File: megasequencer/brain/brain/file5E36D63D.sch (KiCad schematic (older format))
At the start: 24 parts, among them U3 TL074, U4 TL072

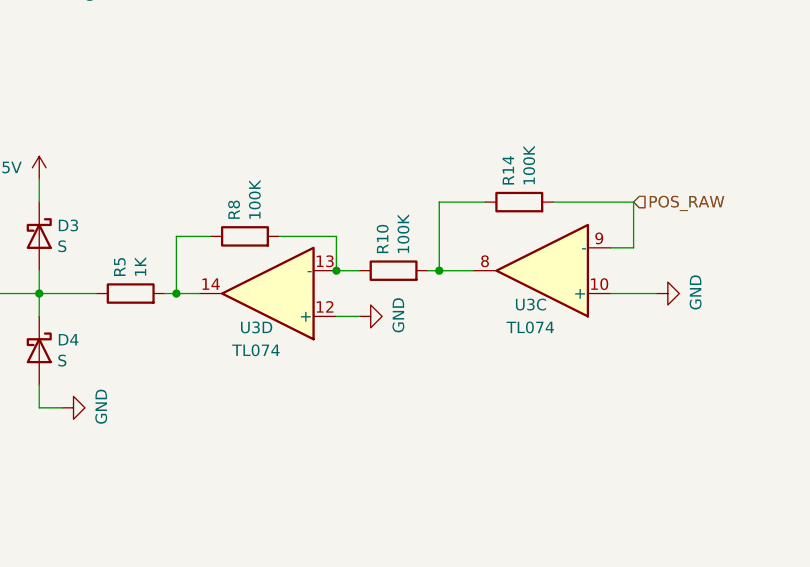
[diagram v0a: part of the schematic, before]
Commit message: Almost done now with both pcbs
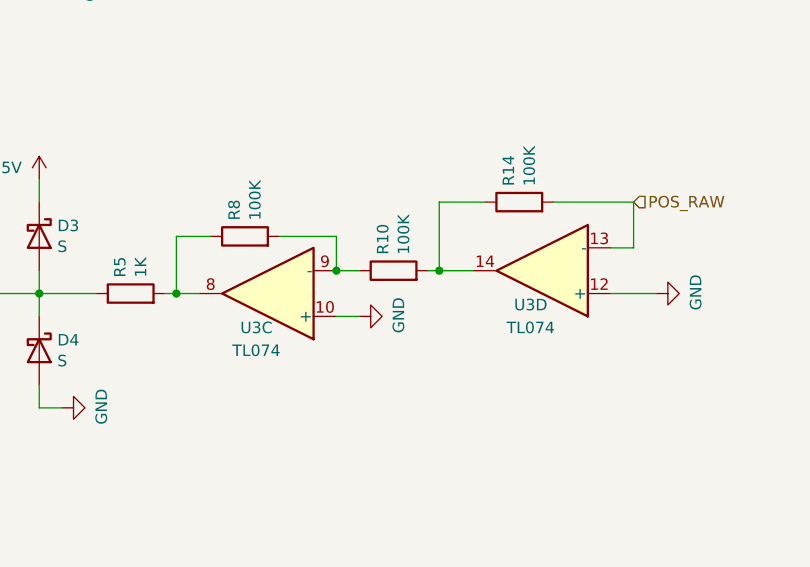
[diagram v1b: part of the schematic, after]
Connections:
- net GND: now also U3.10 (+), U3.12 (+); no longer U3.10 (+), U3.12 (+)
- net POS_RAW: now also U3.13 (-); no longer U3.9 (-)
- net at R10.2, R14.1: now also U3.14; no longer U3.8
- net at R10.1, R8.2: now also U3.9 (-); no longer U3.13 (-)
- net at R5.2, R8.1: now also U3.8; no longer U3.14
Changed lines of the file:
@@
 $Comp
 L Amplifier_Operational:TL074 U?
-U 3 1 5E36F06C
+U 4 1 5E36F06C
 P 3900 4100
 AR Path="/5E36F06C" Ref="U?"  Part="3"
-AR Path="/5E36D63E/5E36F06C" Ref="U3"  Part="3"
+AR Path="/5E36D63E/5E36F06C" Ref="U3"  Part="4"
 F 0 "U3" H 3950 4250 50  0000 C CNN
 F 1 "TL074" H 3950 4350 50  0000 C CNN
 F 2 "Package_DIP:DIP-14_W7.62mm" H 3850 4200 50  0001 C CNN
 F 3 "http://www.ti.com/lit/ds/symlink/tl071.pdf" H 3950 4300 50  0001 C CNN
-	3    3900 4100
+	4    3900 4100
 	-1   0    0    1
 $EndComp
@@
 $Comp
 L Amplifier_Operational:TL074 U?
-U 4 1 5E36F095
+U 3 1 5E36F095
 P 2700 4200
 AR Path="/5E36F095" Ref="U?"  Part="4"
-AR Path="/5E36D63E/5E36F095" Ref="U3"  Part="4"
+AR Path="/5E36D63E/5E36F095" Ref="U3"  Part="3"
 F 0 "U3" H 2750 4350 50  0000 C CNN
 F 1 "TL074" H 2750 4450 50  0000 C CNN
 F 2 "Package_DIP:DIP-14_W7.62mm" H 2650 4300 50  0001 C CNN
 F 3 "http://www.ti.com/lit/ds/symlink/tl071.pdf" H 2750 4400 50  0001 C CNN
-	4    2700 4200
+	3    2700 4200
 	-1   0    0    1
 $EndComp
